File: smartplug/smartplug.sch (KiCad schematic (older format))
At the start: 16 parts

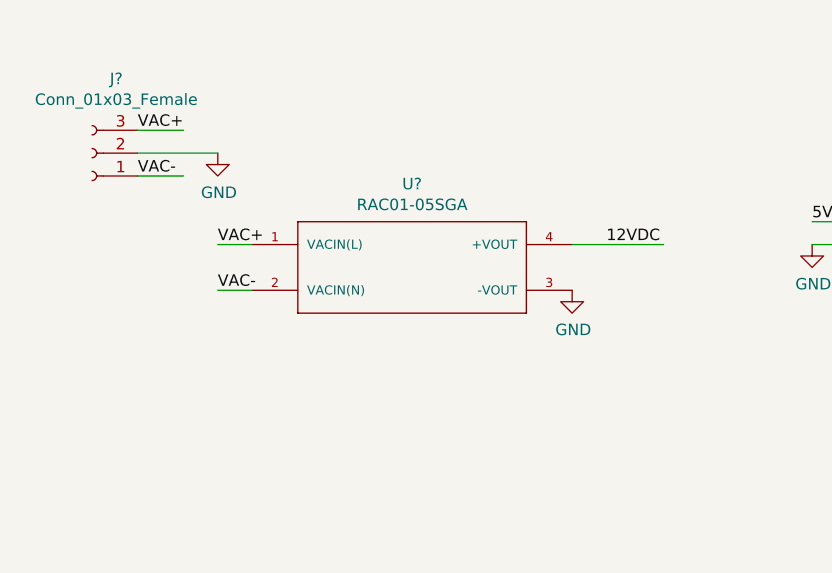
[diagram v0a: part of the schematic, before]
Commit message: added circuit protection
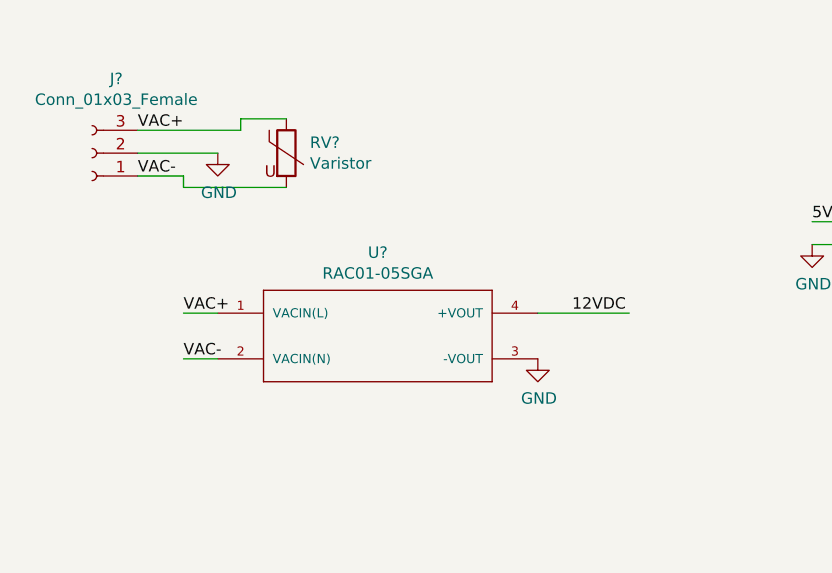
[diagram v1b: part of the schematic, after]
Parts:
- added RV?: Varistor, symbol Device:Varistor
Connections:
- wire segments 39 -> 43
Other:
- moved on the sheet: U?
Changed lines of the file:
@@
 EESchema Schematic File Version 4
 LIBS:smartplug-cache
-LIBS:USBCharger-cache
 EELAYER 26 0
 EELAYER END
@@
 L smartplug-rescue:RAC01-05SGA-RAC01-05SGA U?
 U 1 1 5C93137A
-P 2550 2400
-F 0 "U?" H 2550 2765 50  0000 C CNN
-F 1 "RAC01-05SGA" H 2550 2674 50  0000 C CNN
-F 2 "CONV_RAC01-05SGA" H 2550 2400 50  0001 L BNN
-F 3 "RAC01-05SGA" H 2550 2400 50  0001 L BNN
-F 4 "DIP-4 Recom Power" H 2550 2400 50  0001 L BNN "Field4"
-F 5 "Unavailable" H 2550 2400 50  0001 L BNN "Field5"
-F 6 "RAC01 Series Single Output 5 V 1 W POWERLINE AC/DC Converter" H 2550 2400 50  0001 L BNN "Field6"
-F 7 "Recom Power" H 2550 2400 50  0001 L BNN "Field7"
-F 8 "None" H 2550 2400 50  0001 L BNN "Field8"
-	1    2550 2400
+P 2400 2700
+F 0 "U?" H 2400 3065 50  0000 C CNN
+F 1 "RAC01-05SGA" H 2400 2974 50  0000 C CNN
+F 2 "CONV_RAC01-05SGA" H 2400 2700 50  0001 L BNN
+F 3 "RAC01-05SGA" H 2400 2700 50  0001 L BNN
+F 4 "DIP-4 Recom Power" H 2400 2700 50  0001 L BNN "Field4"
+F 5 "Unavailable" H 2400 2700 50  0001 L BNN "Field5"
+F 6 "RAC01 Series Single Output 5 V 1 W POWERLINE AC/DC Converter" H 2400 2700 50  0001 L BNN "Field6"
+F 7 "Recom Power" H 2400 2700 50  0001 L BNN "Field7"
+F 8 "None" H 2400 2700 50  0001 L BNN "Field8"
+	1    2400 2700
 	1    0    0    -1
 $EndComp
@@
 L power:GND #PWR0103
 U 1 1 5C940AA6
-P 3250 2500
-F 0 "#PWR0103" H 3250 2250 50  0001 C CNN
-F 1 "GND" H 3255 2327 50  0000 C CNN
-F 2 "" H 3250 2500 50  0001 C CNN
-F 3 "" H 3250 2500 50  0001 C CNN
-	1    3250 2500
-	1    0    0    -1
-$EndComp
-Wire Wire Line
-	3250 2300 3650 2300
-Text Label 3400 2300 0    50   ~ 0
+P 3100 2800
+F 0 "#PWR0103" H 3100 2550 50  0001 C CNN
+F 1 "GND" H 3105 2627 50  0000 C CNN
+F 2 "" H 3100 2800 50  0001 C CNN
+F 3 "" H 3100 2800 50  0001 C CNN
+	1    3100 2800
+	1    0    0    -1
+$EndComp
+Wire Wire Line
+	3100 2600 3500 2600
+Text Label 3250 2600 0    50   ~ 0
 12VDC
 $Comp
@@
 	6050 2800 6500 2800
 Wire Wire Line
-	1350 1800 1550 1800
-Wire Wire Line
 	1350 1900 1700 1900
 Wire Wire Line
@@
 VAC-
 Wire Wire Line
-	1850 2300 1700 2300
-Wire Wire Line
-	1850 2500 1700 2500
-Text Label 1700 2300 0    50   ~ 0
+	1700 2600 1550 2600
+Wire Wire Line
+	1700 2800 1550 2800
+Text Label 1550 2600 0    50   ~ 0
 VAC+
-Text Label 1700 2500 0    50   ~ 0
+Text Label 1550 2800 0    50   ~ 0
 VAC-
 $Comp
@@
 Text Label 4300 2200 0    50   ~ 0
 5VDC
+$Comp
+L Device:Varistor RV?
+U 1 1 5CA44C84
+P 2000 1900
+F 0 "RV?" H 2103 1946 50  0000 L CNN
+F 1 "Varistor" H 2103 1855 50  0000 L CNN
+F 2 "" V 1930 1900 50  0001 C CNN
+F 3 "~" H 2000 1900 50  0001 C CNN
+	1    2000 1900
+	1    0    0    -1
+$EndComp
+Wire Wire Line
+	1800 1800 1800 1750
+Wire Wire Line
+	1800 1750 2000 1750
+Wire Wire Line
+	1350 1800 1800 1800
+Wire Wire Line
+	1550 2000 1550 2050
+Wire Wire Line
+	1550 2050 2000 2050
 $EndSCHEMATC
